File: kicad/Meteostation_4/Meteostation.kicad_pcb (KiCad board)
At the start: 2 copper layers, 44 x 44 mm, 113 parts, among them J1 TxD, J10 GM+, J11 GM-, J12 SWD, J13 SWC, J14 ST7735S_CS, J15 OLED_SCL, J16 OLED_SDA, J17 ST7735S_DC, J18 ST7735S_RESET, J2 RxD, J3 BME280_SCL, J4 BME280_SDA, J5 +EXT, J6 +EXT, J7 -EXT, J8 mosi, J9 sclk, Q1 5N10, Q2 IRLML6346, Q3 Q_NPN_BEC, T1 HY931147C, U1 STM32F103C8Tx, U2 LMR50410XDBVR, U3 AD8541, Y2 ECS-250-20-33 25MHz

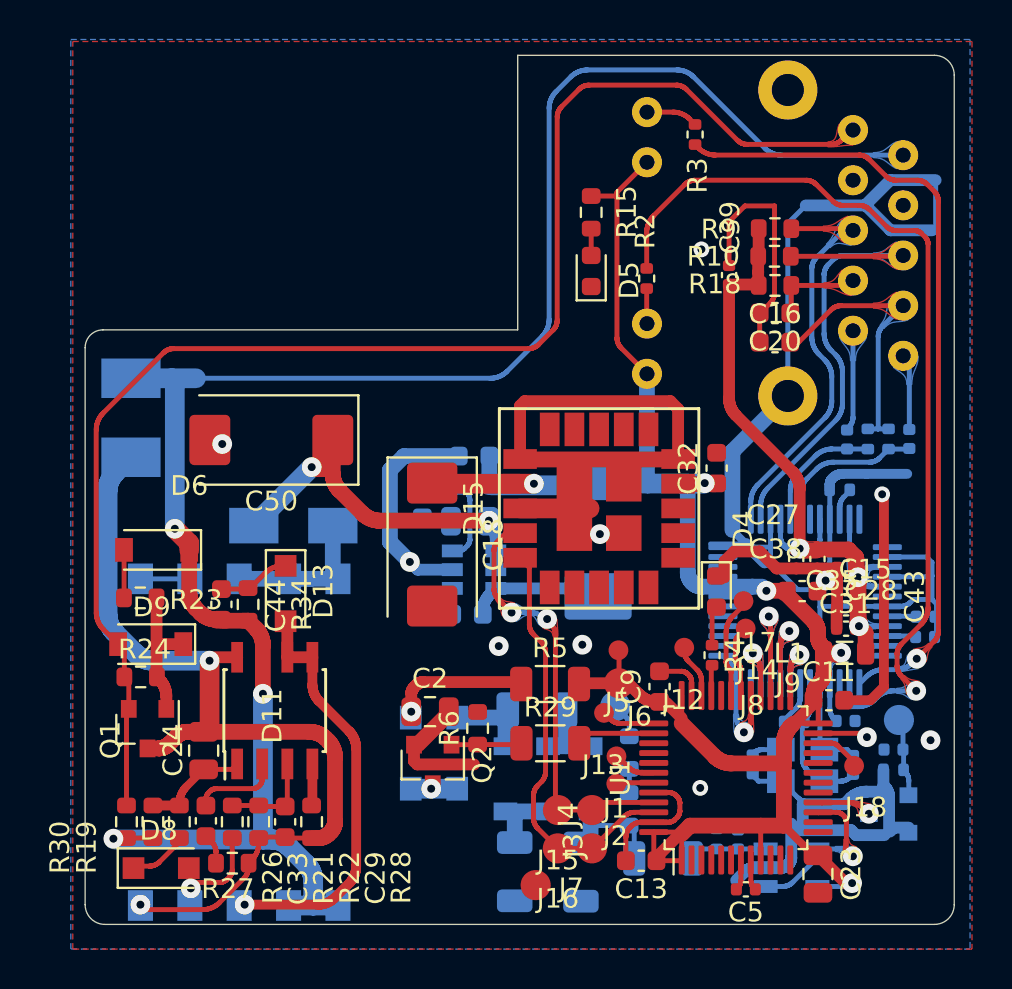
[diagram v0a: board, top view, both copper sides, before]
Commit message: изменено:      FreeCAD/GM_case.FCStd 	изменено:      kicad/BME280/BME280.kicad_pcb 	изменено:      kicad/Meteostation_4/Meteostation-rescue.lib 	изменено:      kicad/Meteostation_4/Meteostation.kicad_pcb 	изменено:      stm32cubeide/Meteostation/.settings/language.settings.xml 	изменено:      stm32cubeide/Meteostation/Core/Inc/main.h 	изменено:      stm32cubeide/Meteostation/Core/Src/main.c 	изменено:      stm32cubeide/Meteostation/Meteostation.ioc 	изменено:      stm32cubeide/Meteostation/Meteostation.launch 	изменено:      stm32cubeide/Meteostation/Release/Core/Src/main.o 	изменено:      stm32cubeide/Meteostation/Release/Core/Src/main.su 	изменено:      stm32cubeide/Meteostation/Release/Core/Src/stm32f1xx_it.o 	изменено:      stm32cubeide/Meteostation/Release/Meteostation.bin 	изменено:      stm32cubeide/Meteostation/Release/Meteostation.elf 	изменено:      stm32cubeide/Meteostation/Release/Meteostation.hex 	изменено:      stm32cubeide/Meteostation/Release/Meteostation.list 	изменено:      stm32cubeide/Meteostation/Release/Meteostation.map
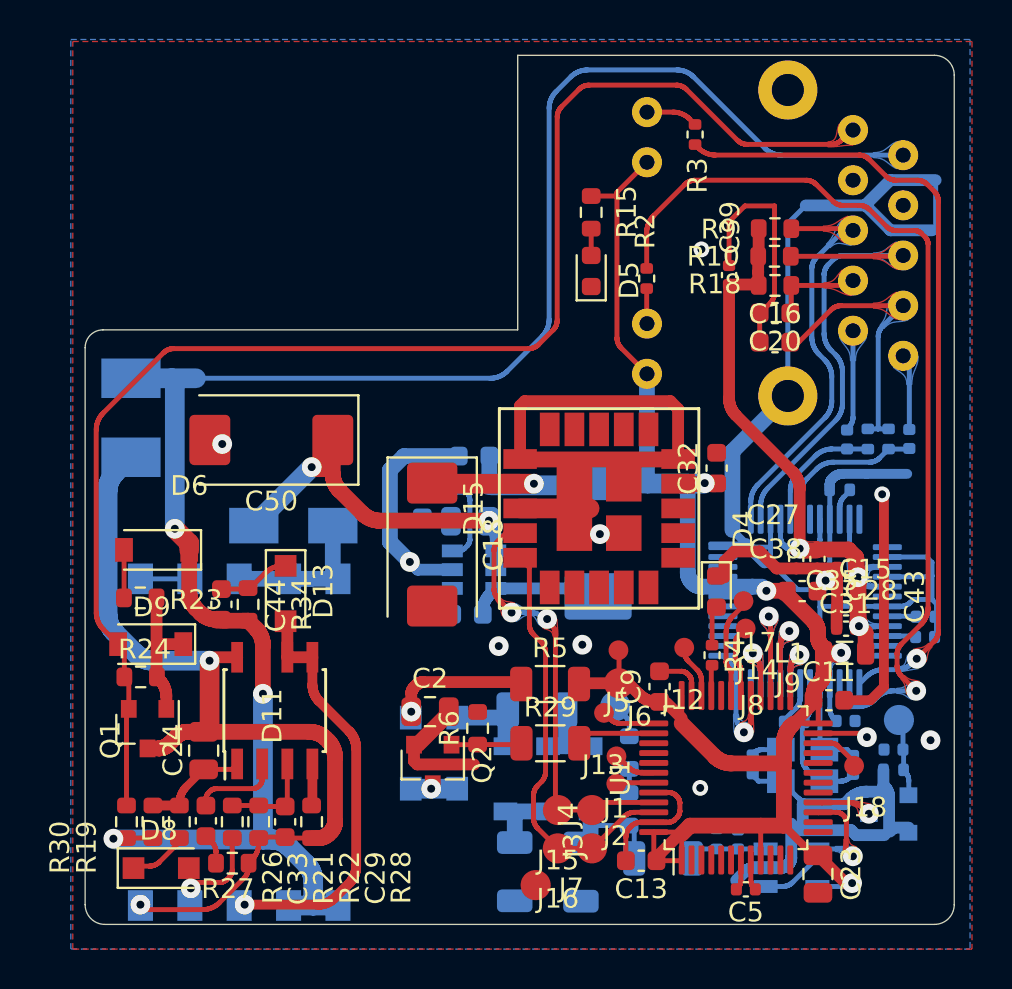
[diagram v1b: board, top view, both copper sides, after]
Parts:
- R7: value 3.4k -> 51k
- R8: value 1.02k -> 22.1k
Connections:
- D3 pad 12: (no net) -> unconnected-(D3-Pad12)
- D3 pad 13: (no net) -> unconnected-(D3-Pad13)
- D3 pad 18: (no net) -> unconnected-(D3-Pad18)
- D3 pad 23: (no net) -> unconnected-(D3-Pad23)
- D3 pad 24: (no net) -> unconnected-(D3-Pad24)
- D3 pad 26: (no net) -> unconnected-(D3-Pad26)
- D3 pad 36: (no net) -> unconnected-(D3-Pad36)
- D3 pad 38: (no net) -> unconnected-(D3-Pad38)
- D3 pad 39: (no net) -> unconnected-(D3-Pad39)
- D3 pad 40: (no net) -> unconnected-(D3-Pad40)
- D3 pad 41: (no net) -> unconnected-(D3-Pad41)
- D3 pad 42: (no net) -> unconnected-(D3-Pad42)
- D3 pad 46: (no net) -> unconnected-(D3-Pad46)
- D3 pad 47: (no net) -> unconnected-(D3-Pad47)
- D3 pad 7: (no net) -> unconnected-(D3-Pad7)
- U1 pad 10: (no net) -> unconnected-(U1-Pad10)
- U1 pad 11: (no net) -> unconnected-(U1-Pad11)
- U1 pad 12: (no net) -> unconnected-(U1-Pad12)
- U1 pad 13: (no net) -> unconnected-(U1-Pad13)
- U1 pad 14: (no net) -> unconnected-(U1-Pad14)
- U1 pad 17: (no net) -> unconnected-(U1-Pad17)
- U1 pad 18: (no net) -> unconnected-(U1-Pad18)
- U1 pad 19: (no net) -> unconnected-(U1-Pad19)
- U1 pad 2: (no net) -> unconnected-(U1-Pad2)
- U1 pad 20: (no net) -> unconnected-(U1-Pad20)
- U1 pad 21: (no net) -> unconnected-(U1-Pad21)
- U1 pad 3: (no net) -> unconnected-(U1-Pad3)
- U1 pad 32: (no net) -> unconnected-(U1-Pad32)
- U1 pad 39: (no net) -> unconnected-(U1-Pad39)
- U1 pad 4: (no net) -> unconnected-(U1-Pad4)
- U1 pad 40: (no net) -> unconnected-(U1-Pad40)
- U1 pad 41: (no net) -> unconnected-(U1-Pad41)
- U1 pad 5: (no net) -> unconnected-(U1-Pad5)
- U1 pad 6: (no net) -> unconnected-(U1-Pad6)
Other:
- net class Default removed
